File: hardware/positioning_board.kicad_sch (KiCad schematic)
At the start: 30 parts, among them J1 4P4C, J2 USB_C_Receptacle_USB2.0_16P, J3 Conn_01x04, J4 Conn_01x05, J5 Conn_01x05, Q1 MMBT3904, Q2 MMBT3904, SW1 SW_Push, SW2 SW_Push, U1 SN65HVD1782DR, U2 CH340K, U3 ESP32-S3-WROOM-1, U4 LSM6DS3

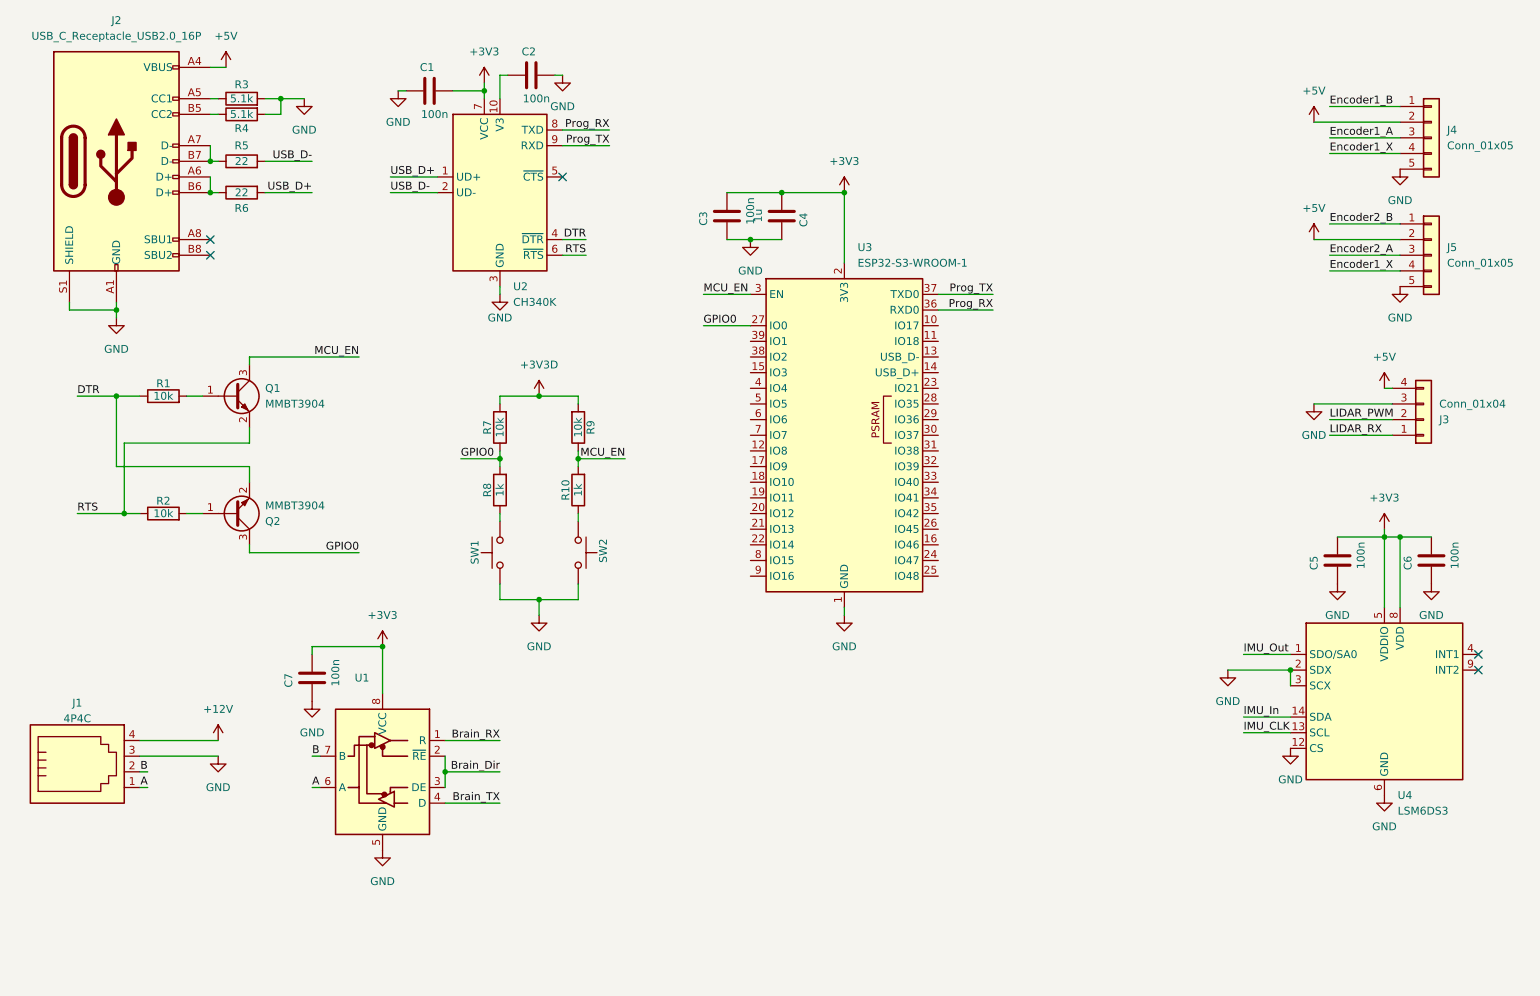
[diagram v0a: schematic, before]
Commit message: feat: draft layout
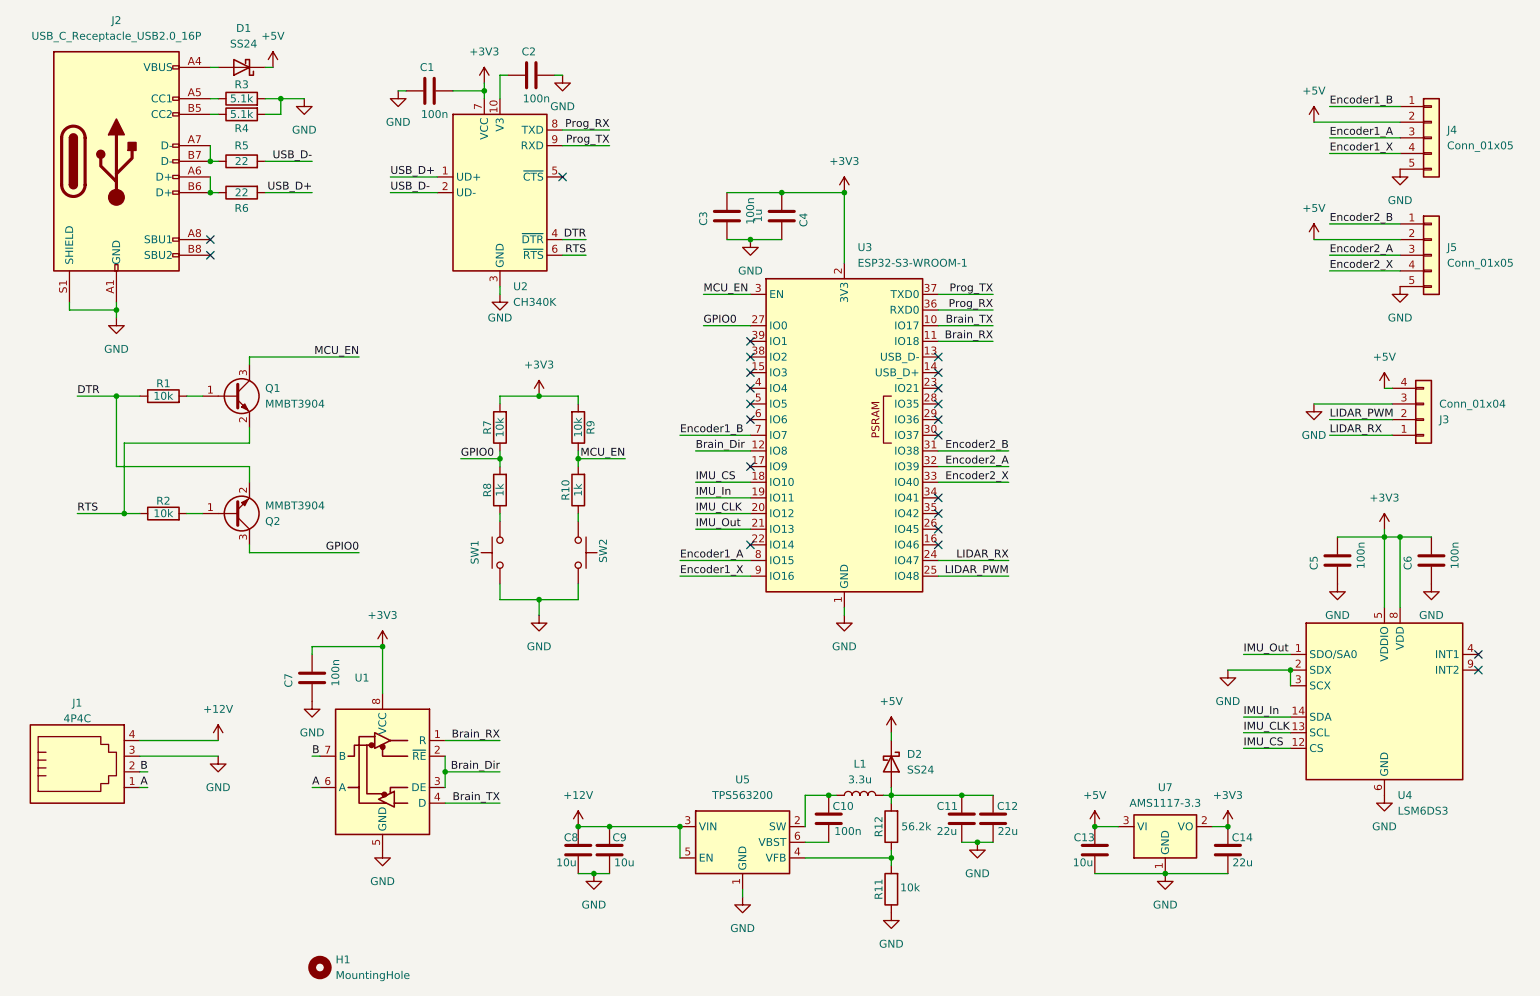
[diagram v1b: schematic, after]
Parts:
- added C10: 100n, Capacitor_SMD:C_0603_1608Metric, symbol Device:C
- added C11, C12, C14: 22u, Capacitor_SMD:C_0603_1608Metric, symbol Device:C
- added C13, C8, C9: 10u, Capacitor_SMD:C_0603_1608Metric, symbol Device:C
- added D1, D2: SS24, Diode_SMD:D_SMA, symbol Diode:SS24
- added H1: MountingHole, MountingHole:MountingHole_3.2mm_M3, symbol Mechanical:MountingHole
- added L1: 3.3u, Inductor_SMD:L_Changjiang_FXL0630, symbol Device:L
- added R11: 10k, Resistor_SMD:R_0603_1608Metric, symbol Device:R
- added R12: 56.2k, Resistor_SMD:R_0603_1608Metric, symbol Device:R
- added U5: TPS563200, Package_TO_SOT_SMD:SOT-23-6, symbol Regulator_Switching:TPS563200
- added U7: AMS1117-3.3, Package_TO_SOT_SMD:SOT-223-3_TabPin2, symbol Regulator_Linear:AMS1117-3.3
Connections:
- net +3V3D is gone; now on net +3V3: R7.2, R9.2
- net +12V: now also C8.2, C9.2, U5.3 (VIN), U5.5 (EN)
- net +3V3: now also C14.2, U7.2 (VO)
- net +5V: now also C13.2, D1.1 (K), D2.1 (K), U7.3 (VI); no longer J2.A4 (VBUS), J2.A9 (VBUS), J2.B4 (VBUS), J2.B9 (VBUS)
- net Brain_Dir: now also U3.12 (IO8)
- net Brain_RX: now also U3.11 (IO18)
- net Brain_TX: now also U3.10 (IO17)
- net Encoder1_A: now also U3.8 (IO15)
- net Encoder1_B: now also U3.7 (IO7)
- net Encoder1_X: now also U3.9 (IO16); no longer J5.4 (Pin_4)
- net Encoder2_A: now also U3.32 (IO39)
- net Encoder2_B: now also U3.31 (IO38)
- net GND: now also C11.1, C12.1, C13.1, C14.1, C8.1, C9.1, R11.1, U5.1 (GND), U7.1 (GND); no longer U4.12 (CS)
- net IMU_CLK: now also U3.20 (IO12)
- net IMU_In: now also U3.19 (IO11)
- net IMU_Out: now also U3.21 (IO13)
- net LIDAR_PWM: now also U3.25 (IO48)
- net LIDAR_RX: now also U3.24 (IO47)
- net IMU_CS: now reaches U3.18 (IO10)
- net IMU_CS: now also U4.12 (CS)
- net Encoder2_X: now reaches U3.33 (IO40)
- net Encoder2_X: now also J5.4 (Pin_4)
- new net: C10.2, L1.1, U5.2 (SW)
- new net: R11.2, R12.1, U5.4 (VFB)
- new net: C10.1, U5.6 (VBST)
- new net: D1.2 (A), J2.A4 (VBUS), J2.A9 (VBUS), J2.B4 (VBUS), J2.B9 (VBUS)
- new net: C11.2, C12.2, D2.2 (A), L1.2, R12.2
- no-connect marks 5 -> 23
